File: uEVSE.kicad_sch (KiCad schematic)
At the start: 27 parts, among them J1 12VDC input, J2 GSsP, J3 PE/CP, J4 Ss(B), U1 NE555P, U2 LM358

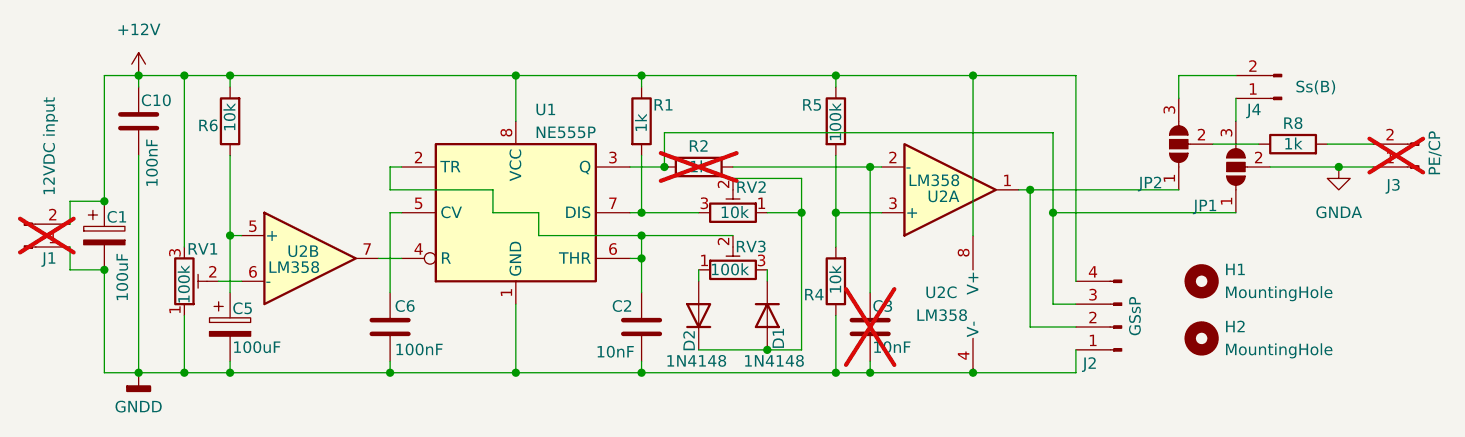
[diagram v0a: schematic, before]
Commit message: Add files via upload
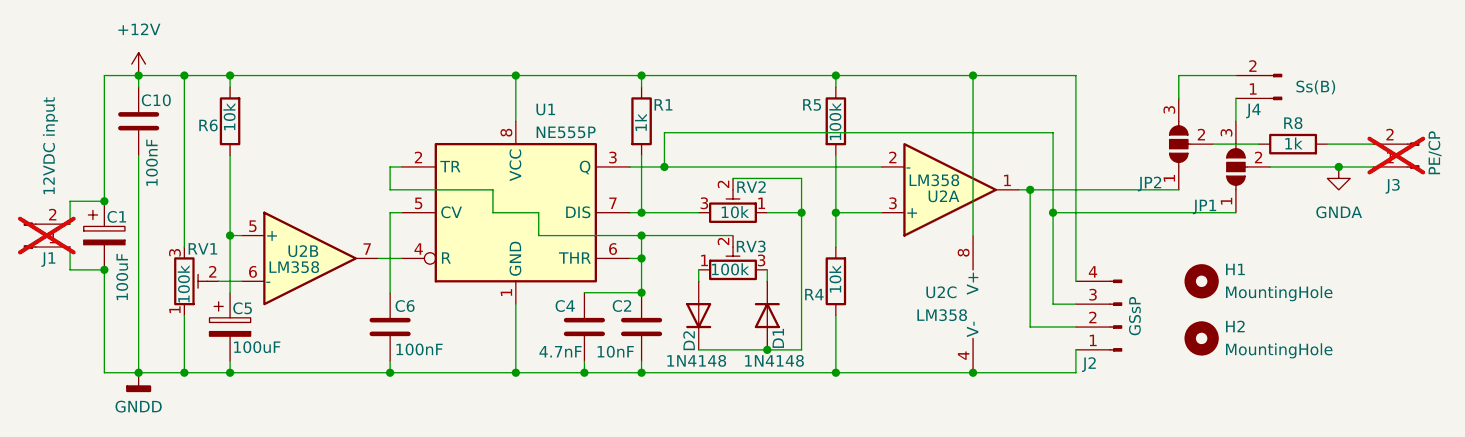
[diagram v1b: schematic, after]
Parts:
- removed C3: 10nF, Capacitor_THT:C_Rect_L7.0mm_W2.5mm_P5.00mm, symbol Device:C
- removed R2: 1k, Resistor_THT:R_Axial_DIN0207_L6.3mm_D2.5mm_P2.54mm_Vertical, symbol Device:R
- added C4: 4.7nF, Capacitor_THT:C_Rect_L7.0mm_W2.5mm_P5.00mm, symbol Device:C
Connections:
- net GNDD: now also C4.2
- net at J2.3 (Pin_3), JP1.1 (A), U1.3 (Q): now also U2.2 (-)
- net at C2.1, RV3.2, U1.2 (TR)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: now also C4.1
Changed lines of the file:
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@@
+	)
+	(junction
+		(at 99.06 40.64)
+		(diameter 0)
+		(color 0 0 0 0)
 	)
 	(junction
@@
 	)
 	(junction
+		(at 90.17 63.5)
+		(diameter 0)
+		(color 0 0 0 0)
+	)
+	(junction
+		(at 96.52 54.61)
+		(diameter 0)
+		(color 0 0 0 0)
+	)
+	(junction
 		(at 82.55 63.5)
 		(diameter 0)
@@
 	)
 	(junction
-		(at 121.92 40.64)
-		(diameter 0)
-		(color 0 0 0 0)
-	)
-	(junction
-		(at 121.92 63.5)
-		(diameter 0)
-		(color 0 0 0 0)
-	)
-	(junction
 		(at 45.72 63.5)
 		(diameter 0)
@@
 		(color 0 0 0 0)
 	)
-	(junction
-		(at 99.06 40.64)
-		(diameter 0)
-		(color 0 0 0 0)
-	)
 	(wire
 		(pts
@@
 	(wire
 		(pts
+			(xy 99.06 40.64) (xy 123.19 40.64)
+		)
+		(stroke
+			(width 0)
+			(type default)
+		)
+	)
+	(wire
+		(pts
 			(xy 118.11 45.72) (xy 123.19 45.72)
 		)
@@
 	(wire
 		(pts
-			(xy 121.92 40.64) (xy 121.92 54.61)
-		)
-		(stroke
-			(width 0)
-			(type default)
-		)
-	)
-	(wire
-		(pts
-			(xy 121.92 63.5) (xy 133.35 63.5)
-		)
-		(stroke
-			(width 0)
-			(type default)
-		)
-	)
-	(wire
-		(pts
 			(xy 142.24 45.72) (xy 162.56 45.72)
 		)
@@
 	(wire
 		(pts
+			(xy 90.17 54.61) (xy 96.52 54.61)
+		)
+		(stroke
+			(width 0)
+			(type default)
+		)
+	)
+	(wire
+		(pts
 			(xy 110.49 45.72) (xy 114.3 45.72)
 		)
@@
 	(wire
 		(pts
+			(xy 90.17 63.5) (xy 96.52 63.5)
+		)
+		(stroke
+			(width 0)
+			(type default)
+		)
+	)
+	(wire
+		(pts
 			(xy 142.24 45.72) (xy 142.24 55.88)
 		)
@@
 	(wire
 		(pts
+			(xy 90.17 62.23) (xy 90.17 63.5)
+		)
+		(stroke
+			(width 0)
+			(type default)
+		)
+	)
+	(wire
+		(pts
 			(xy 68.58 43.18) (xy 80.01 43.18)
 		)
@@
 	(wire
 		(pts
-			(xy 121.92 62.23) (xy 121.92 63.5)
-		)
-		(stroke
-			(width 0)
-			(type default)
-		)
-	)
-	(wire
-		(pts
 			(xy 162.56 30.48) (xy 156.21 30.48)
 		)
@@
 	(wire
 		(pts
-			(xy 106.68 40.64) (xy 121.92 40.64)
-		)
-		(stroke
-			(width 0)
-			(type default)
-		)
-	)
-	(wire
-		(pts
-			(xy 118.11 63.5) (xy 121.92 63.5)
+			(xy 118.11 63.5) (xy 133.35 63.5)
 		)
 		(stroke
@@
 	(wire
 		(pts
-			(xy 82.55 63.5) (xy 96.52 63.5)
+			(xy 82.55 63.5) (xy 90.17 63.5)
 		)
 		(stroke
@@
 		(pts
 			(xy 40.64 63.5) (xy 45.72 63.5)
-		)
-		(stroke
-			(width 0)
-			(type default)
-		)
-	)
-	(wire
-		(pts
-			(xy 121.92 40.64) (xy 123.19 40.64)
 		)
 		(stroke
@@
 	)
 	(symbol
-		(lib_id "Device:R")
-		(at 102.87 40.64 90)
-		(unit 1)
-		(exclude_from_sim no)
-		(in_bom no)
-		(on_board yes)
-		(dnp yes)
-		(property "Reference" "R2"
-			(at 102.87 38.354 90)
-			(effects
-				(font
-					(size 1.27 1.27)
-				)
-			)
-		)
-		(property "Value" "1k"
-			(at 102.87 40.64 90)
-			(effects
-				(font
-					(size 1.27 1.27)
-				)
-			)
-		)
-		(property "Footprint" "Resistor_THT:R_Axial_DIN0207_L6.3mm_D2.5mm_P2.54mm_Vertical"
-			(at 102.87 42.418 90)
-			(effects
-				(font
-					(size 1.27 1.27)
-				)
-				(hide yes)
-			)
-		)
-		(property "Datasheet" "~"
-			(at 102.87 40.64 0)
-			(effects
-				(font
-					(size 1.27 1.27)
-				)
-				(hide yes)
-			)
-		)
-		(property "Description" "Resistor"
-			(at 102.87 40.64 0)
-			(effects
-				(font
-					(size 1.27 1.27)
-				)
-				(hide yes)
-			)
-		)
-		(pin "1"
-		)
-		(pin "2"
-		)
-		(instances
-			(project "uEVSE"
-				(path "/9cd33690-2e07-4508-ba14-37821b89d687"
-					(reference "R2")
-					(unit 1)
-				)
-			)
-		)
-	)
-	(symbol
 		(lib_id "Device:C_Polarized")
 		(at 36.83 48.26 0)
@@
 	)
 	(symbol
-		(lib_id "Device:C")
-		(at 121.92 58.42 0)
-		(unit 1)
-		(exclude_from_sim no)
-		(in_bom no)
-		(on_board yes)
-		(dnp yes)
-		(property "Reference" "C3"
-			(at 122.174 56.134 0)
-			(effects
-				(font
-					(size 1.27 1.27)
-				)
-				(justify left)
-			)
-		)
-		(property "Value" "10nF"
-			(at 122.174 60.706 0)
-			(effects
-				(font
-					(size 1.27 1.27)
-				)
-				(justify left)
-			)
-		)
-		(property "Footprint" "Capacitor_THT:C_Rect_L7.0mm_W2.5mm_P5.00mm"
-			(at 122.8852 62.23 0)
-			(effects
-				(font
-					(size 1.27 1.27)
-				)
-				(hide yes)
-			)
-		)
-		(property "Datasheet" "~"
-			(at 121.92 58.42 0)
-			(effects
-				(font
-					(size 1.27 1.27)
-				)
-				(hide yes)
-			)
-		)
-		(property "Description" "Unpolarized capacitor"
-			(at 121.92 58.42 0)
-			(effects
-				(font
-					(size 1.27 1.27)
-				)
-				(hide yes)
-			)
-		)
-		(pin "1"
-		)
-		(pin "2"
-		)
-		(instances
-			(project "uEVSE"
-				(path "/9cd33690-2e07-4508-ba14-37821b89d687"
-					(reference "C3")
-					(unit 1)
-				)
-			)
-		)
-	)
-	(symbol
 		(lib_id "Connector:Conn_01x02_Pin")
 		(at 167.64 33.02 180)
@@
 					(unit 1)
 				)
+			)
+		)
+	)
+	(symbol
+		(lib_id "Device:C")
+		(at 90.17 58.42 0)
+		(unit 1)
+		(exclude_from_sim no)
+		(in_bom yes)
+		(on_board yes)
+		(dnp no)
+		(property "Reference" "C4"
+			(at 86.868 56.134 0)
+			(effects
+				(font
+					(size 1.27 1.27)
+				)
+				(justify left)
+			)
+		)
+		(property "Value" "4.7nF"
+			(at 85.09 61.214 0)
+			(effects
+				(font
+					(size 1.27 1.27)
+				)
+				(justify left)
+			)
+		)
+		(property "Footprint" "Capacitor_THT:C_Rect_L7.0mm_W2.5mm_P5.00mm"
+			(at 91.1352 62.23 0)
+			(effects
+				(font
+					(size 1.27 1.27)
+				)
+				(hide yes)
+			)
+		)
+		(property "Datasheet" "~"
+			(at 90.17 58.42 0)
+			(effects
+				(font
+					(size 1.27 1.27)
+				)
+				(hide yes)
+			)
+		)
+		(property "Description" "Unpolarized capacitor"
+			(at 90.17 58.42 0)
+			(effects
+				(font
+					(size 1.27 1.27)
+				)
+				(hide yes)
+			)
+		)
+		(pin "1"
+		)
+		(pin "2"
+		)
+		(instances
+			(project "uEVSE"
+				(path "/9cd33690-2e07-4508-ba14-37821b89d687"
+					(reference "C4")
+					(unit 1)
+				)
